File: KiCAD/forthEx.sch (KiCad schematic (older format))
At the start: 58 parts, among them CON1 SD_Card, CON2 BARREL_JACK 2,1mm, J1 RCA_JACK, J2 RCA_JACK, J3 RJ12, P1 ICSP, Q1 2N3906, Q2 2N3904, SW1 Power, SW2 reset, U1 LD1117v33, U2 LM7805CT, U3 PIC24EP512GP202, U4 25LC1024, U5 23LC1024, X1 8Mhz

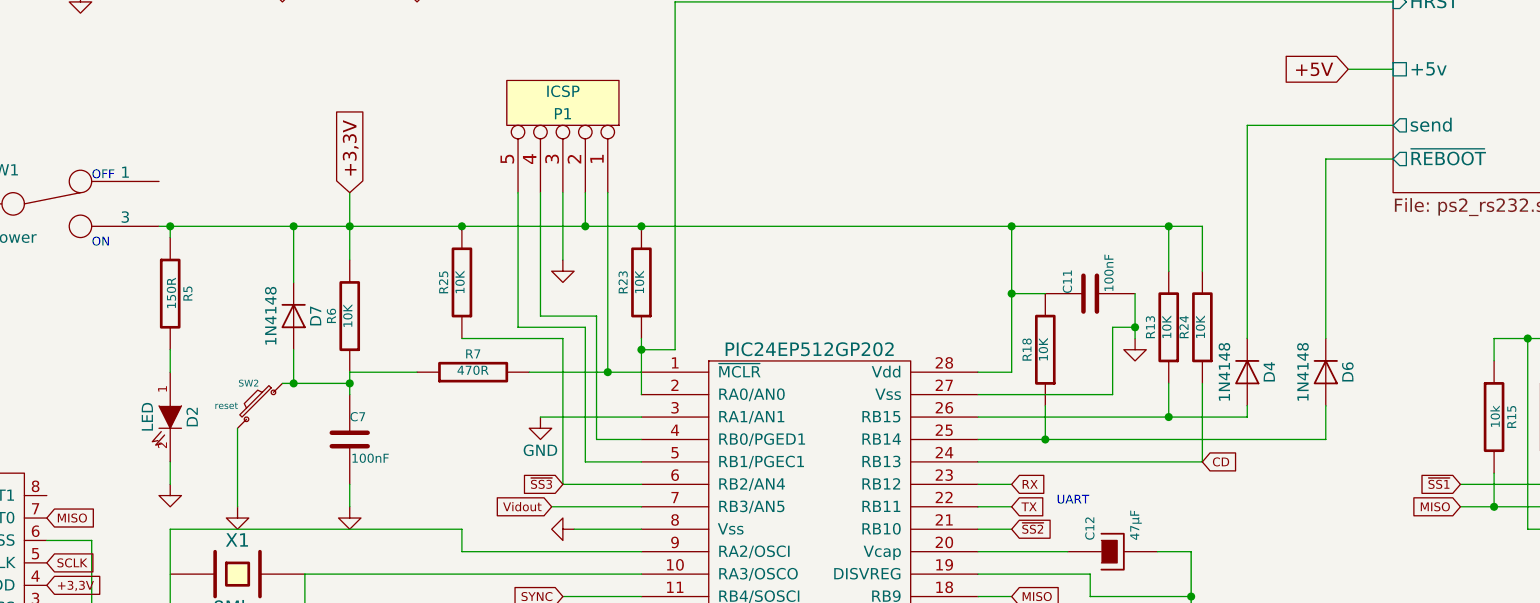
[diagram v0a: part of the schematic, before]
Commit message: réorganisation projet
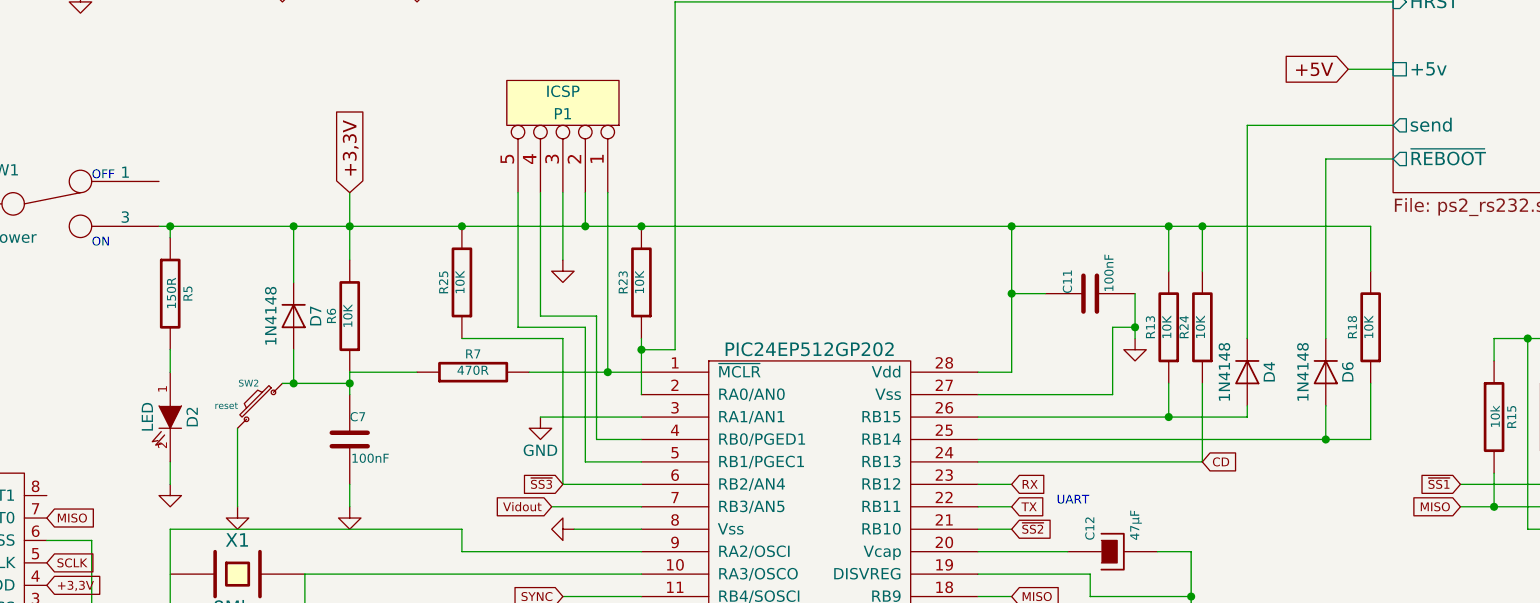
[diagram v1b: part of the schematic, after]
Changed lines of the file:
@@
 NoConn ~ 750  5850
-$Comp
-L R-RESCUE-forthEx R18
-U 1 1 5873EBF4
-P 7000 2950
-F 0 "R18" V 7080 2950 40  0000 C CNN
-F 1 "10K" V 7007 2951 40  0000 C CNN
-F 2 "~" V 6930 2950 30  0000 C CNN
-F 3 "~" H 7000 2950 30  0000 C CNN
-	1    7000 2950
-	-1   0    0    1
-$EndComp
 $Comp
 L R R14
@@
 	8350 1700 8550 1700
 Wire Wire Line
-	3050 2400 7700 2400
+	3050 2400 8450 2400
 Wire Wire Line
 	7900 3250 7900 3200
@@
 	5200 6850 5600 6850
 Wire Wire Line
-	6700 3350 8250 3350
-Wire Wire Line
 	4850 4150 4850 4250
 Connection ~ 4850 4250
 Wire Wire Line
 	5150 4150 5200 4150
-Wire Wire Line
-	7000 3350 7000 3200
 $Comp
 L GND #PWR17
@@
 	1    0    0    -1
 $EndComp
-$Comp
-L D D6
-U 1 1 58740C49
-P 8250 3050
-F 0 "D6" H 8250 3150 50  0000 C CNN
-F 1 "1N4148" H 8250 2950 50  0000 C CNN
-F 2 "" H 8250 3050 50  0000 C CNN
-F 3 "" H 8250 3050 50  0000 C CNN
-	1    8250 3050
-	0    1    1    0
-$EndComp
-Wire Wire Line
-	8250 3350 8250 3200
-Connection ~ 7000 3350
-Wire Wire Line
-	8250 2900 8250 2100
 Wire Wire Line
 	8250 2100 8550 2100
@@
 	3650 2950 3650 3100
 Connection ~ 3650 3100
+$Comp
+L D D6
+U 1 1 58897471
+P 8250 3050
+F 0 "D6" H 8250 3150 50  0000 C CNN
+F 1 "1N4148" H 8250 2950 50  0000 C CNN
+F 2 "" H 8250 3050 50  0000 C CNN
+F 3 "" H 8250 3050 50  0000 C CNN
+	1    8250 3050
+	0    1    1    0
+$EndComp
+Wire Wire Line
+	8250 2100 8250 2900
+Wire Wire Line
+	8250 3200 8250 3350
+Wire Wire Line
+	6700 3350 8450 3350
+$Comp
+L R-RESCUE-forthEx R18
+U 1 1 588977AF
+P 8450 2850
+F 0 "R18" V 8530 2850 40  0000 C CNN
+F 1 "10K" V 8457 2851 40  0000 C CNN
+F 2 "~" V 8380 2850 30  0000 C CNN
+F 3 "~" H 8450 2850 30  0000 C CNN
+	1    8450 2850
+	-1   0    0    1
+$EndComp
+Wire Wire Line
+	8450 2400 8450 2600
+Connection ~ 7700 2400
+Wire Wire Line
+	8450 3350 8450 3100
+Connection ~ 8250 3350
 $EndSCHEMATC
